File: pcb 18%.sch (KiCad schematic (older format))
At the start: 33 parts, among them SW1 SW_Push, U1 ATmega32U4-AU, Y1 16MHz

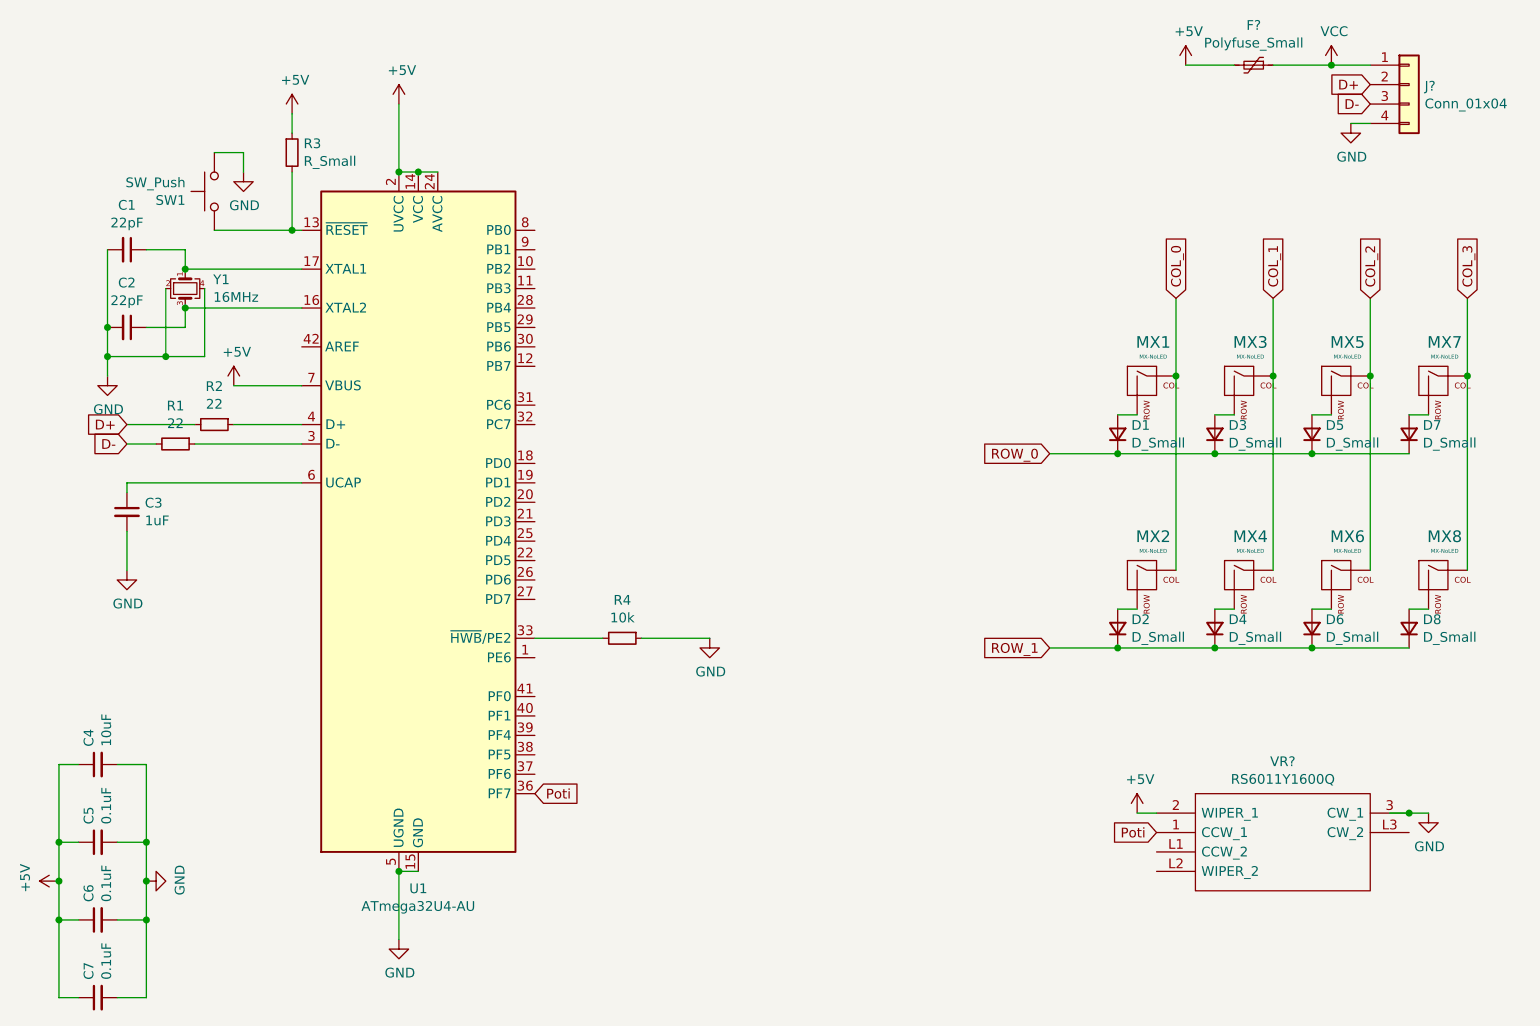
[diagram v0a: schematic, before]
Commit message: diesdas
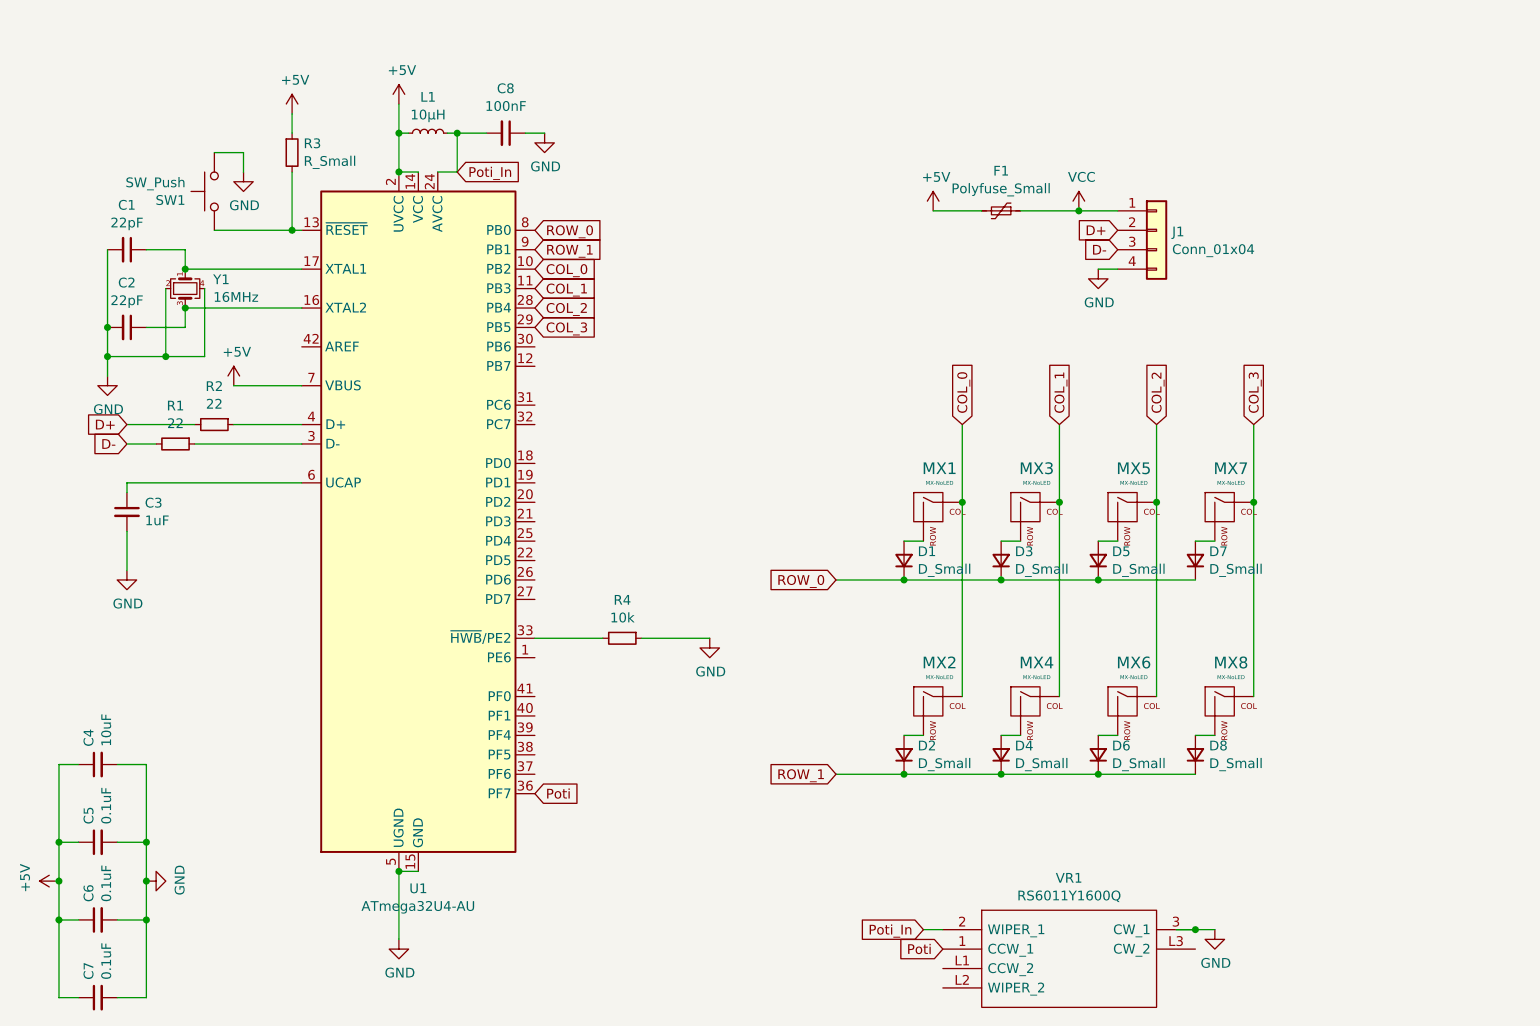
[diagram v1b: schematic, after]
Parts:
- added C8: 100nF, Capacitor_SMD:C_0805_2012Metric, symbol Device:C_Small
- added L1: 10μH, symbol Device:L_Small
- J1: renamed from J?; footprint (none) -> random-keyboard-parts:JST-SR-4
- VR1: renamed from VR?; footprint RS6011Y1600Q -> RS6011Y1600Q:RS6011Y1600Q
- gave numbers to parts that had none: 1
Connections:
- net +5V: now also L1.1; no longer U1.24 (AVCC), U1.44 (AVCC), VR1.2 (WIPER_1)
- net COL_0: now also U1.10 (PB2)
- net COL_1: now also U1.11 (PB3)
- net COL_2: now also U1.28 (PB4)
- net COL_3: now also U1.29 (PB5)
- net GND: now also C8.1
- net ROW_0: now also U1.8 (PB0)
- net ROW_1: now also U1.9 (PB1)
- new net Poti_In: C8.2, L1.2, U1.24 (AVCC), U1.44 (AVCC), VR1.2 (WIPER_1)
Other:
- moved on the sheet: D1, D2, D3, D4, D5, D6, D7, D8, F1, J1, MX1, MX2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
